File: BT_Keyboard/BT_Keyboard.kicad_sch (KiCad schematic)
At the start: 161 parts, among them J1 Conn_01x22_Pin, J2 Conn_01x22_Pin, J3 Conn_01x14_Pin, J4 Conn_01x22_Pin, J5 Conn_01x22_Pin, SW1 SW_Push_45deg, SW10 SW_Push_45deg, SW11 SW_Push_45deg, SW12 SW_Push_45deg, SW13 SW_Push_45deg, SW14 SW_Push_45deg, SW15 SW_Push_45deg, SW16 SW_Push_45deg, SW17 SW_Push_45deg, SW18 SW_Push_45deg, SW19 SW_Push_45deg, SW2 SW_Push_45deg, SW20 SW_Push_45deg, SW21 SW_Push_45deg, SW22 SW_Push_45deg, SW23 SW_Push_45deg, SW24 SW_Push_45deg, SW25 SW_Push_45deg, SW26 SW_Push_45deg, SW27 SW_Push_45deg, SW28 Backspace, SW29 Tab, SW3 SW_Push_45deg, SW30 Cap, SW31 SW_Push_45deg, SW32 SW_Push_45deg, SW33 SW_Push_45deg, SW34 SW_Push_45deg, SW35 SW_Push_45deg, SW36 SW_Push_45deg, SW37 SW_Push_45deg, SW38 SW_Push_45deg, SW39 SW_Push_45deg, SW4 SW_Push_45deg, SW40 SW_Push_45deg, SW41 SW_Push_45deg, SW42 SW_Push_45deg, SW43 SW_Push_45deg, SW44 SW_Push_45deg, SW45 SW_Push_45deg, SW46 SW_Push_45deg, SW47 SW_Push_45deg, SW48 SW_Push_45deg, SW49 SW_Push_45deg, SW5 SW_Push_45deg, SW50 SW_Push_45deg, SW51 SW_Push_45deg, SW52 SW_Push_45deg, SW53 SW_Push_45deg, SW54 Enter, SW55 SW_Push_45deg, SW56 Shift, SW57 SW_Push_45deg, SW58 SW_Push_45deg, SW59 SW_Push_45deg, SW6 SW_Push_45deg, SW60 SW_Push_45deg, SW61 SW_Push_45deg, SW62 SW_Push_45deg, SW63 SW_Push_45deg, SW64 SW_Push_45deg, SW65 SW_Push_45deg, SW66 SW_Push_45deg, SW67 SW_Push_45deg, SW68 SW_Push_45deg, SW69 SW_Push_45deg, SW7 SW_Push_45deg, SW70 SW_Push_45deg, SW71 SW_Push_45deg, SW72 SW_Push_45deg, SW73 SW_Push_45deg, SW74 SW_Push_45deg, SW75 SW_Push_45deg, SW76 SW_Push_45deg, SW77 SW_Push_45deg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

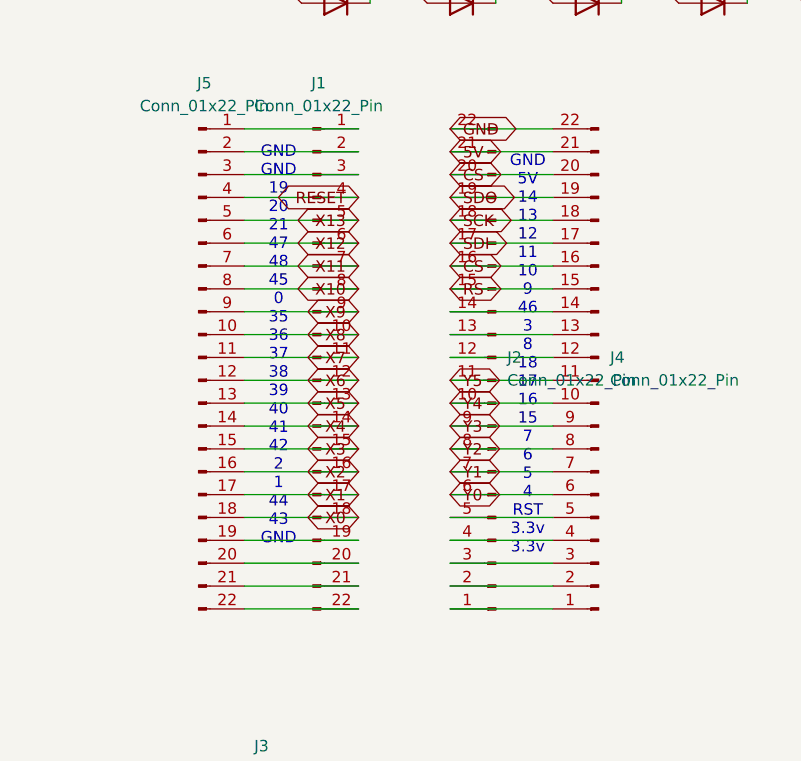
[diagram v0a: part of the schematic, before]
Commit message: Add files via upload
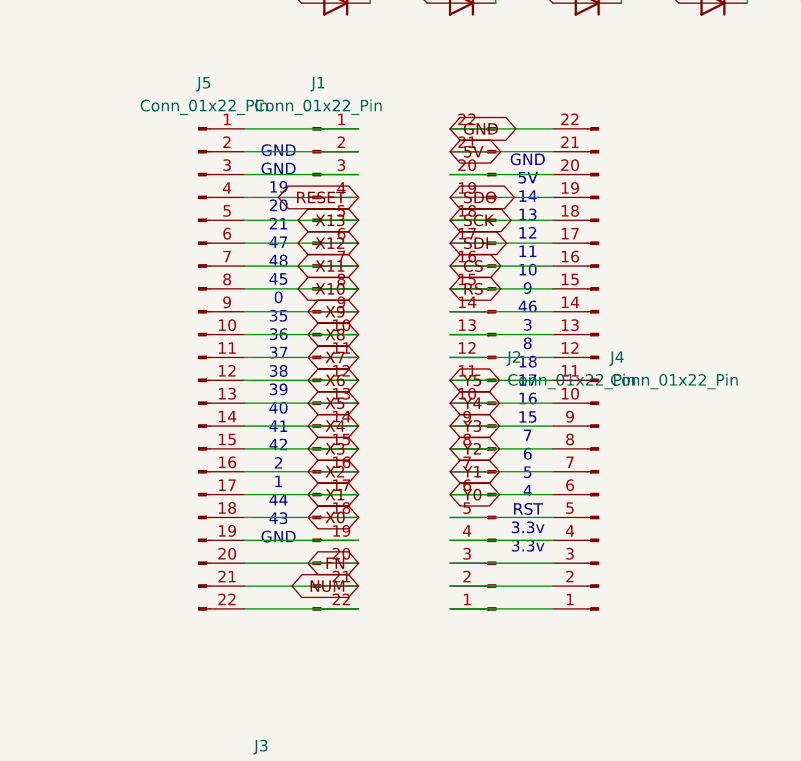
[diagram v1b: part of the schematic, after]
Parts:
- removed D55: 1N4001, Diode_THT:D_DO-41_SOD81_P10.16mm_Horizontal, symbol Diode:1N4001
- removed SW55: SW_Push_45deg, Button_Switch_Keyboard:SW_Cherry_MX_1.00u_PCB, symbol Switch:SW_Push_45deg
- added D42: 1N4001, Diode_THT:D_DO-41_SOD81_P10.16mm_Horizontal, symbol Diode:1N4001
- added SW42: SW_Push_45deg, Button_Switch_Keyboard:SW_Cherry_MX_1.00u_PCB, symbol Switch:SW_Push_45deg
- renumbered D31 to D30, D33 to D31, D35 to D32, D37 to D33, D39 to D34, D41 to D35, D43 to D36, D45 to D37, D47 to D38, D49 to D39, D51 to D40, D53 to D41, D30 to D43, D32 to D44, D34 to D45, D36 to D46, D38 to D47, D40 to D48, D42 to D49, D44 to D50, D46 to D51, D48 to D52, D50 to D53, D52 to D54, D54 to D55, SW31 to SW30, SW33 to SW31, SW35 to SW32, SW37 to SW33, SW39 to SW34, SW41 to SW35, SW43 to SW36, SW45 to SW37, SW47 to SW38, SW49 to SW39, SW51 to SW40, SW53 to SW41, SW30 to SW43, SW32 to SW44, SW34 to SW45, SW36 to SW46, SW38 to SW47, SW40 to SW48, SW42 to SW49, SW44 to SW50, SW46 to SW51, SW48 to SW52, SW50 to SW53, SW52 to SW54, SW54 to SW55
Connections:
- net CS: no longer J2.20 (Pin_20), J4.20 (Pin_20)
- net FN: now also J1.20 (Pin_20), J5.20 (Pin_20)
- net NUM: now also J1.21 (Pin_21), J5.21 (Pin_21)
- net X13: now also D42.1 (K)
- net Y2: now also SW42.1
- new net: J2.20 (Pin_20), J4.20 (Pin_20)
- new net: D42.2 (A), SW42.2

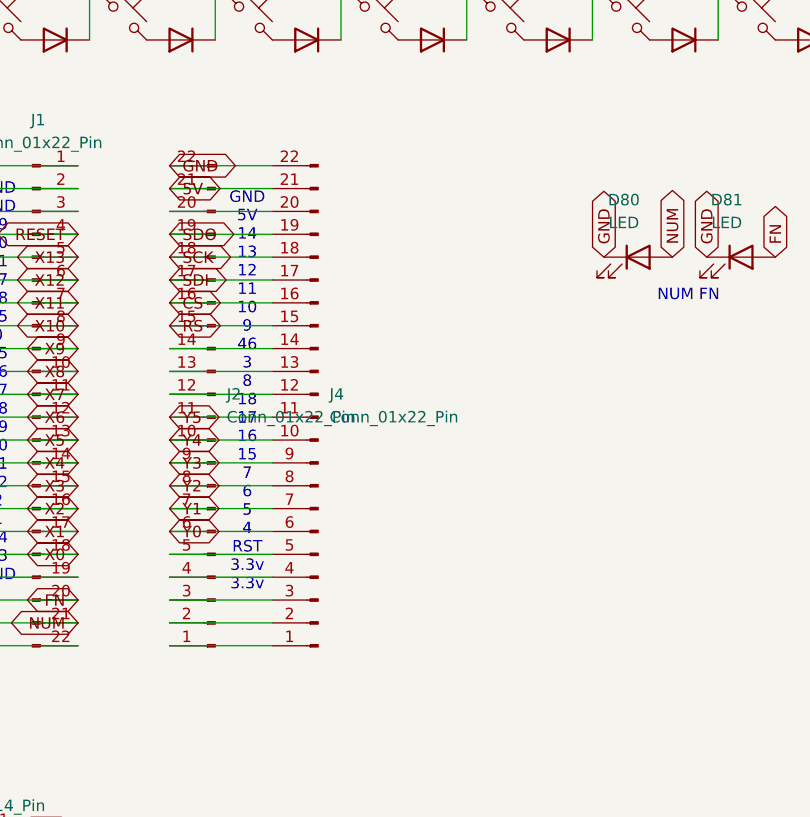
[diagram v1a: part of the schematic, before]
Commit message: Add files via upload
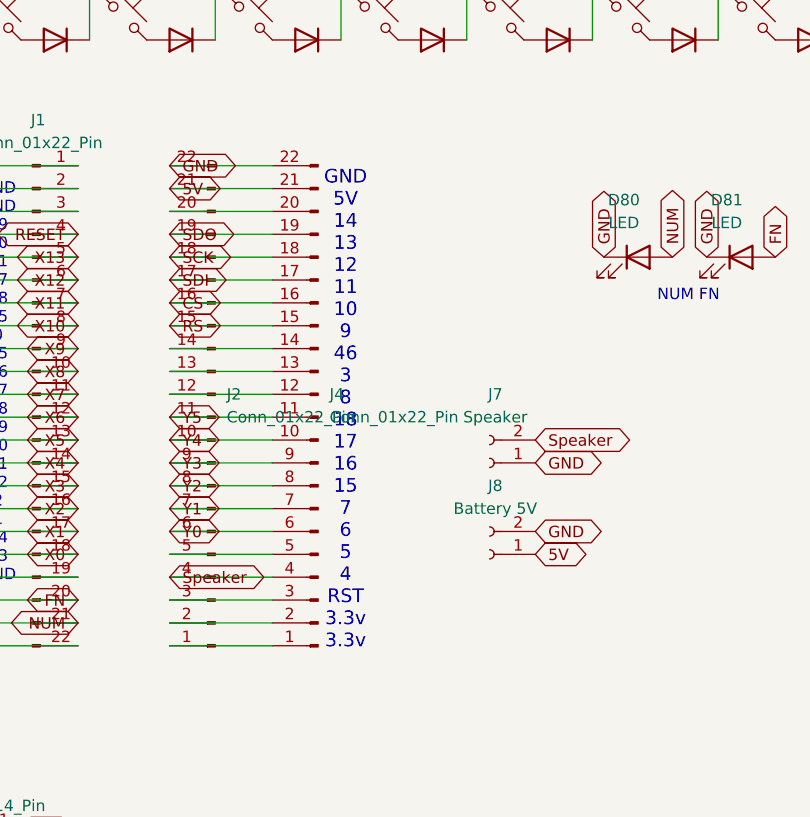
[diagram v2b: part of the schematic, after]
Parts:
- added J7: Speaker, Connector_PinSocket_2.54mm:PinSocket_1x02_P2.54mm_Vertical, symbol Connector:Conn_01x02_Socket
- added J8: Battery 5V, Connector_PinSocket_2.54mm:PinSocket_1x02_P2.54mm_Vertical, symbol Connector:Conn_01x02_Socket
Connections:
- net 5V: now also J8.1 (Pin_1)
- net GND: now also J7.1 (Pin_1), J8.2 (Pin_2)
- net Speaker: now reaches J2.4 (Pin_4), J4.4 (Pin_4)
- net Speaker: now also J7.2 (Pin_2)

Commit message: Add files via upload
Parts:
- SW1, SW10, SW11, SW12, SW13, SW14, SW15, SW16, SW17, SW18, SW19, SW2, SW20, SW21, SW22, SW23, SW24, SW25, SW26, SW27, SW3, SW30, SW31, SW32, SW33, SW34, SW35, SW36, SW37, SW38, SW39, SW4, SW40, SW41, SW42, SW44, SW45, SW46, SW47, SW48, SW49, SW5, SW50, SW51, SW52, SW53, SW54, SW57, SW58, SW59, SW6, SW60, SW61, SW62, SW63, SW64, SW65, SW66, SW67, SW68, SW69, SW7, SW70, SW71, SW72, SW73, SW74, SW75, SW76, SW77, SW8, SW9: footprint Button_Switch_Keyboard:SW_Cherry_MX_1.00u_PCB -> PCM_Switch_Keyboard_Hotswap_Kailh:SW_Hotswap_Kailh_MX_Plated_1.00u
- SW28: footprint Button_Switch_Keyboard:SW_Cherry_MX_1.75u_PCB -> PCM_Switch_Keyboard_Hotswap_Kailh:SW_Hotswap_Kailh_MX_Plated_1.75u
- SW29: footprint Button_Switch_Keyboard:SW_Cherry_MX_1.25u_PCB -> PCM_Switch_Keyboard_Hotswap_Kailh:SW_Hotswap_Kailh_MX_Plated_1.25u
- SW43: footprint Button_Switch_Keyboard:SW_Cherry_MX_1.50u_PCB -> PCM_Switch_Keyboard_Hotswap_Kailh:SW_Hotswap_Kailh_MX_Plated_1.50u
- SW55, SW56: footprint Button_Switch_Keyboard:SW_Cherry_MX_2.00u_PCB -> PCM_Switch_Keyboard_Hotswap_Kailh:SW_Hotswap_Kailh_MX_Plated_2.00u
